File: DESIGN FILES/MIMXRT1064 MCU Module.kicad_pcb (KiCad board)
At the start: 6 copper layers, 60 x 22 mm, 78 parts, among them J601 TF-15x15, U401 MIMXRT1064CVL5B, U601 IS25WP064A-JBLE, U602 IS42S16160J-6BLI, U701 M.2-B-KEY, Y401 7V24000026, Y402 Q13FC1350000200

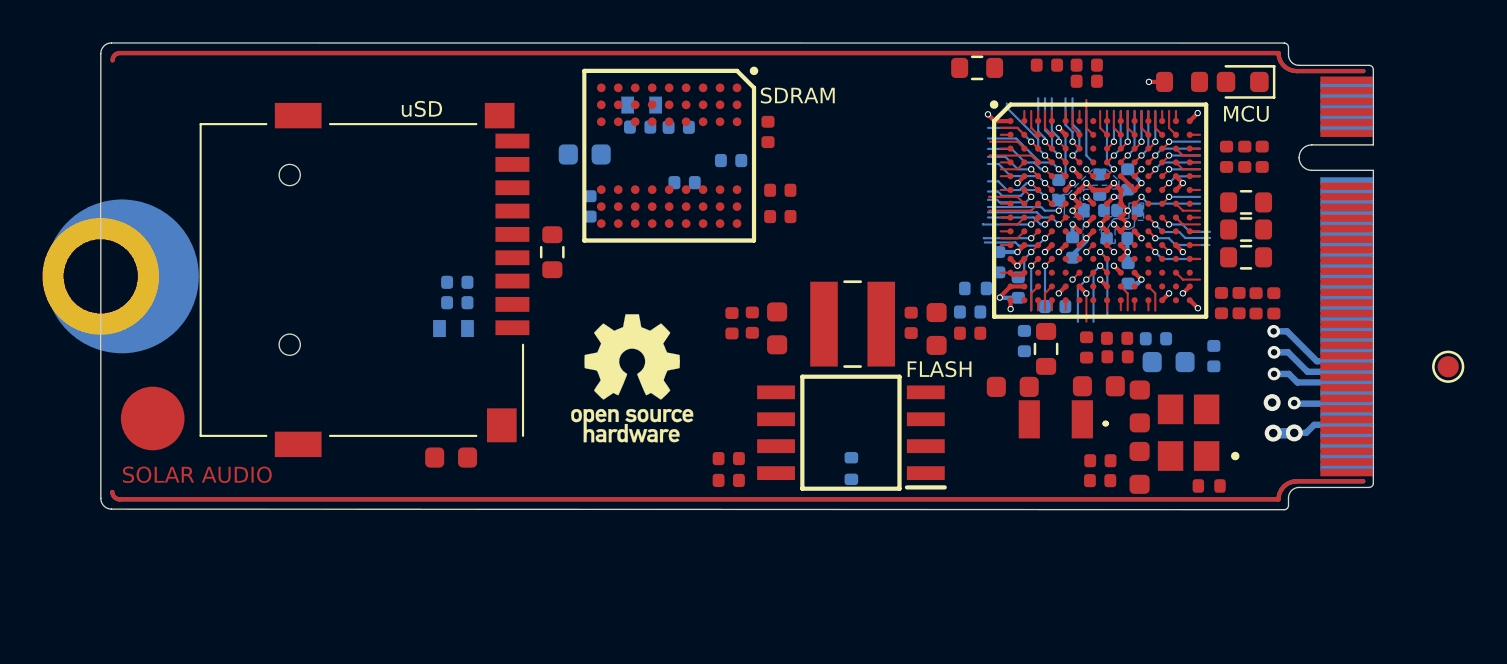
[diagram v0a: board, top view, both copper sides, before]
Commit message: updates
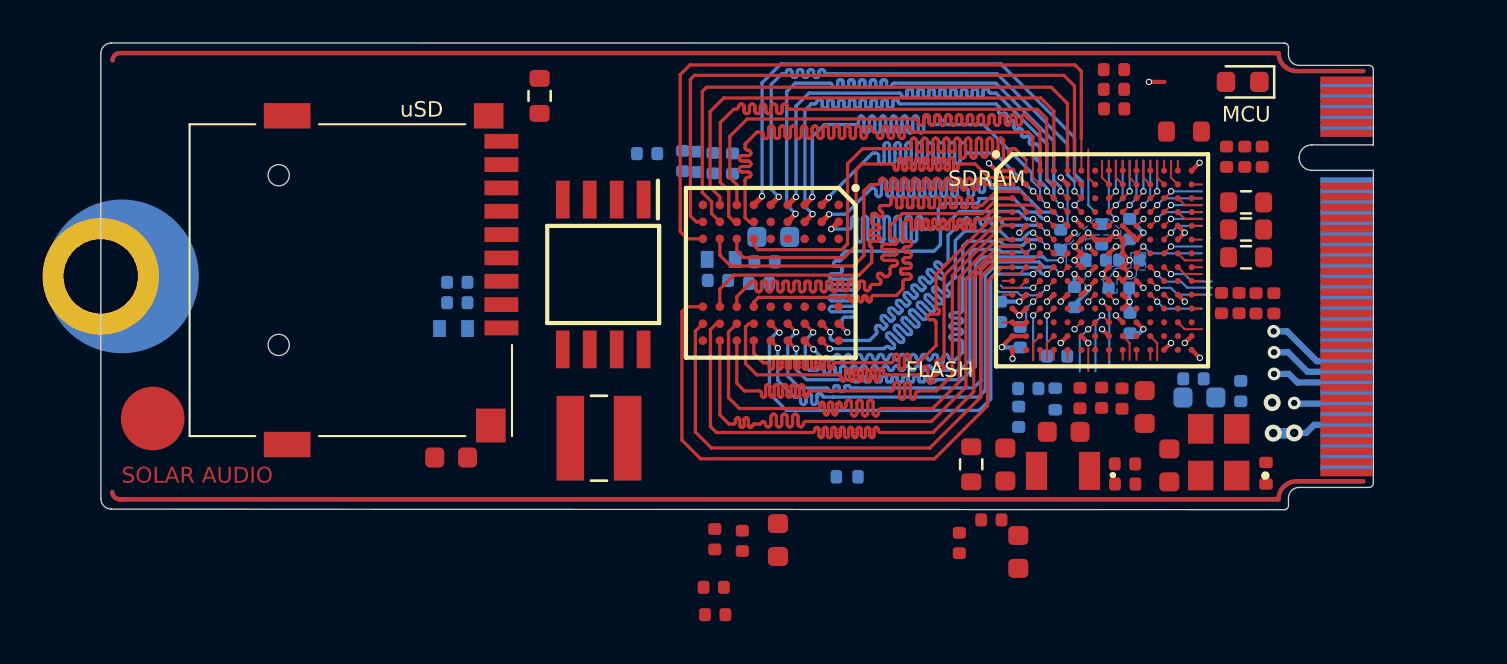
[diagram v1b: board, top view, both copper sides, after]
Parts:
- removed R502: 0R, MY RESISTOR LIBRARY:0603WAF0000T5E
- removed REF**: OSHW-Logo_5.7x6mm_SilkScreen, Symbol:OSHW-Logo_5.7x6mm_SilkScreen
- removed REF**: TestPoint_Pad_D1.0mm, TestPoint:TestPoint_Pad_D1.0mm
- C603, C605, C609: moved to B.Cu
- moved U601 13.9 mm to (142.5, 102.7), turned to -90 degrees
- moved L401 13.1 mm to (142.3, 110.4)
- moved C427 11.2 mm to (162.1, 115.7)
- moved C421 10.6 mm to (159.3, 115.3)
- moved C425 10.3 mm to (149.1, 115.2)
- moved C426 10.2 mm to (147.8, 115.1)
- moved C419 9.98 mm to (150.8, 115.2)
- moved C601 9.70 mm to (150.5, 100.9)
- moved C602 9.26 mm to (149.9, 103.1), turned to 180 degrees
- moved C502 8.86 mm to (160.8, 114.2)
- moved FB601 8.19 mm to (148.1, 102.0), turned to 180 degrees
- moved R501 7.39 mm to (139.5, 94.2)
- moved U602 7.31 mm to (150.4, 102.6)
- moved R503 6.48 mm to (159.9, 111.6), turned to 90 degrees
- moved R403 6.42 mm to (163.8, 108.5), turned to -90 degrees
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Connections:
- U401 pad B3: /MCU GPIO & BUS/SDRAM_CLK_RES -> SDRAM_CLK
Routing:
- net SDRAM_CLK: track 0.00 -> 34.5 mm
- net SDRAM_A4: track 0.47 -> 32.5 mm
- net SDRAM_A1: track 0.47 -> 31.9 mm
- net SDRAM_CKE: track 0.47 -> 30.8 mm
- net SDRAM_A3: track 0.47 -> 30.3 mm
- net SDRAM_BA1: track 0.47 -> 29.5 mm
- net SDRAM_A5: track 1.26 -> 30.3 mm
- net SDRAM_CS: track 0.47 -> 29.2 mm
- net SDRAM_BA0: track 0.47 -> 28.7 mm
- net SDRAM_A12: track 0.47 -> 28.2 mm
- net SDRAM_WE: track 0.47 -> 27.9 mm
- net SDRAM_A10: track 1.80 -> 29.2 mm
- net SDRAM_RAS: track 1.24 -> 28.1 mm
- net SDRAM_A7: track 0.47 -> 27.3 mm
- net SDRAM_A2: track 2.45 -> 28.9 mm
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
